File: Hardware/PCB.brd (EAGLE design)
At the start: 170.4 x 111.2 mm, 102 parts, among them IC1 BD5229G-TR, IC2 XC6220A331MR-G, J1 112A-TAAR-R03_ATTEND, J2 QWIIC_RIGHT_ANGLE, J3 FH34SRJ-24S-0.5SH_99_, J4 SAMACSYS_PARTS_USB4110-GF-A, Q1 20V/4.2A/52mΩ/1.4W, Q2 SI1308EDL-T1-GE3, Q3 20V/4.2A/52mΩ/1.4W, U1 ESP32-C6-WROOM-1-N8, U2 MAX17048G+T10, U3 W25Q512JVEIQ, U4 DS3231SN#

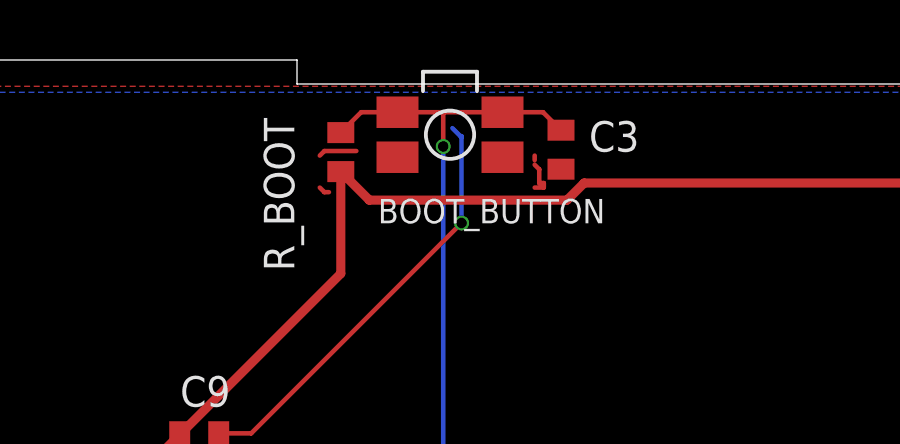
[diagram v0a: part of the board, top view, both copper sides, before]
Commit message: fix issues
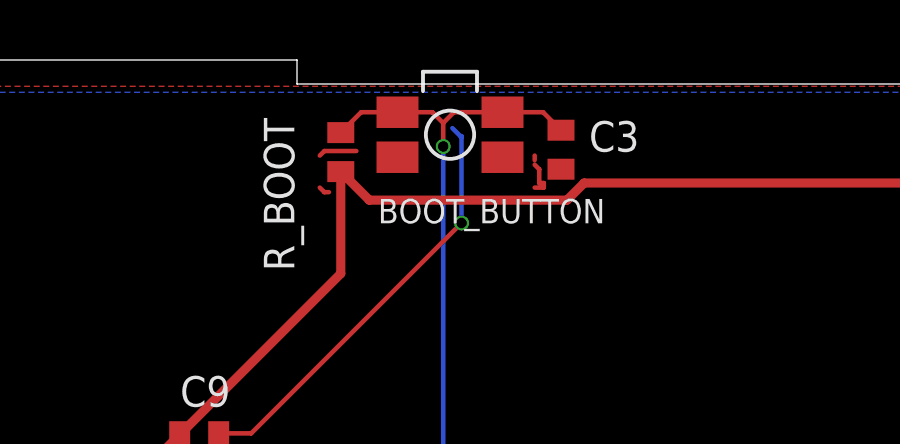
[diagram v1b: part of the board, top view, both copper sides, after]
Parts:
- C25: value 100nF -> 4.7uF
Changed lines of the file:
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@@
 <attribute name="SPICEPREFIX" value="C" x="77.99" y="19.67" size="1.778" layer="27" rot="R270" display="off"/>
 </element>
-<element name="C25" library="DeskAssistant v19 v2" library_urn="urn:adsk.wipprod:fs.file:vf.c-uWg7zGRE2SlFihlENo6g" package="ESP32_WROVER_EAGLE-LTSPICE_C0402" value="100nF" x="148.06" y="52.69" smashed="yes" rot="R270">
+<element name="C25" library="DeskAssistant v19 v2" library_urn="urn:adsk.wipprod:fs.file:vf.c-uWg7zGRE2SlFihlENo6g" package="ESP32_WROVER_EAGLE-LTSPICE_C0402" value="4.7uF" x="148.06" y="52.69" smashed="yes" rot="R270">
 <attribute name="DATASHEET" value="https://ro.mouser.com/datasheet/2/447/KEM_C1006_X5R_SMD-3316465.pdf" x="148.06" y="52.69" size="1.778" layer="27" rot="R270" display="off"/>
 <attribute name="MOUSER_PRICE-STOCK" value="https://ro.mouser.com/ProductDetail/KEMET/C0402C475K8PACTU?qs=sGAEpiMZZMsh%252B1woXyUXj%252BeMYF%2FJh1ZHWLnD7xub%252BoY%3D" x="148.06" y="52.69" size="1.778" layer="27" rot="R270" display="off"/>
@@
 <wire x1="27.7" y1="108.86" x2="27.101" y2="109.459" width="0.1524" layer="1"/>
 <wire x1="27.101" y1="109.459" x2="25.75" y2="109.459" width="0.1524" layer="1"/>
-<wire x1="22.25" y1="109.459" x2="23.7744" y2="109.459" width="0.1524" layer="1"/>
-<wire x1="23.7744" y1="109.459" x2="25.75" y2="109.459" width="0.1524" layer="1"/>
 <wire x1="21.039" y1="109.459" x2="22.25" y2="109.459" width="0.1524" layer="1"/>
 <wire x1="20.36" y1="108.78" x2="21.039" y2="109.459" width="0.1524" layer="1"/>
 <wire x1="23.7744" y1="79.5528" x2="23.7744" y2="71.0184" width="0.1524" layer="1"/>
 <wire x1="23.7744" y1="108.3184" x2="23.7744" y2="79.5528" width="0.1524" layer="16"/>
-<wire x1="23.7744" y1="109.459" x2="23.7744" y2="108.3184" width="0.1524" layer="1"/>
+<wire x1="23.7744" y1="108.3184" x2="23.7744" y2="109.1" width="0.1524" layer="1"/>
 <wire x1="23.7744" y1="71.0184" x2="23.85" y2="70.99" width="0.1524" layer="1"/>
 <via x="23.7744" y="79.5528" extent="1-16" drill="0.35">
@@
 <via x="23.7744" y="108.3184" extent="1-16" drill="0.35">
 </via>
+<wire x1="22.25" y1="109.459" x2="23.4154" y2="109.459" width="0.1524" layer="1"/>
+<wire x1="23.4154" y1="109.459" x2="23.7744" y2="109.1" width="0.1524" layer="1"/>
+<wire x1="23.7744" y1="109.1" x2="24.1334" y2="109.459" width="0.1524" layer="1"/>
+<wire x1="24.1334" y1="109.459" x2="25.75" y2="109.459" width="0.1524" layer="1"/>
 </signal>
 <signal name="VBAT">
